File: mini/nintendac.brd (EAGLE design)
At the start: 30 x 45 mm, 30 parts, among them IC1 STM32F10XCXT6, IC2 REG1117, IC3 24C64ST, X1 USB-MICROB

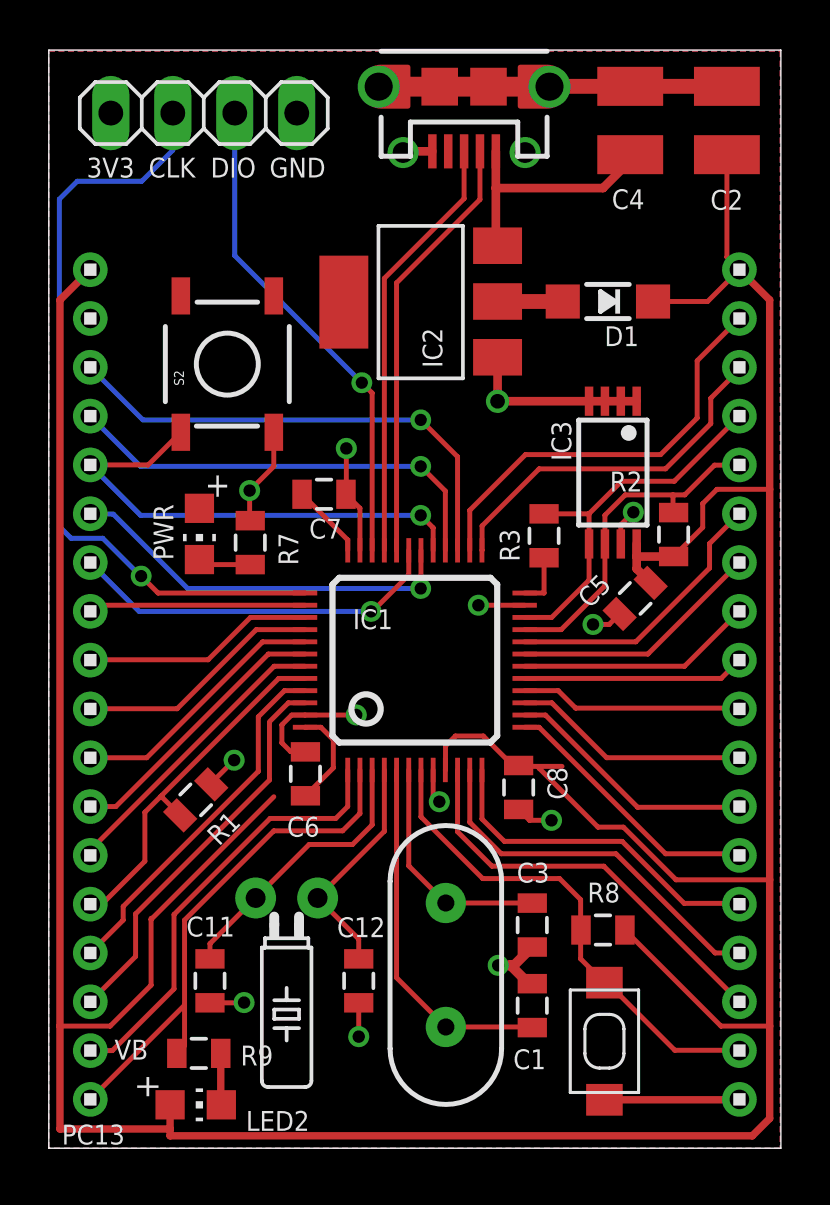
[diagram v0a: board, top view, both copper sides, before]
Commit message: updated mini layout
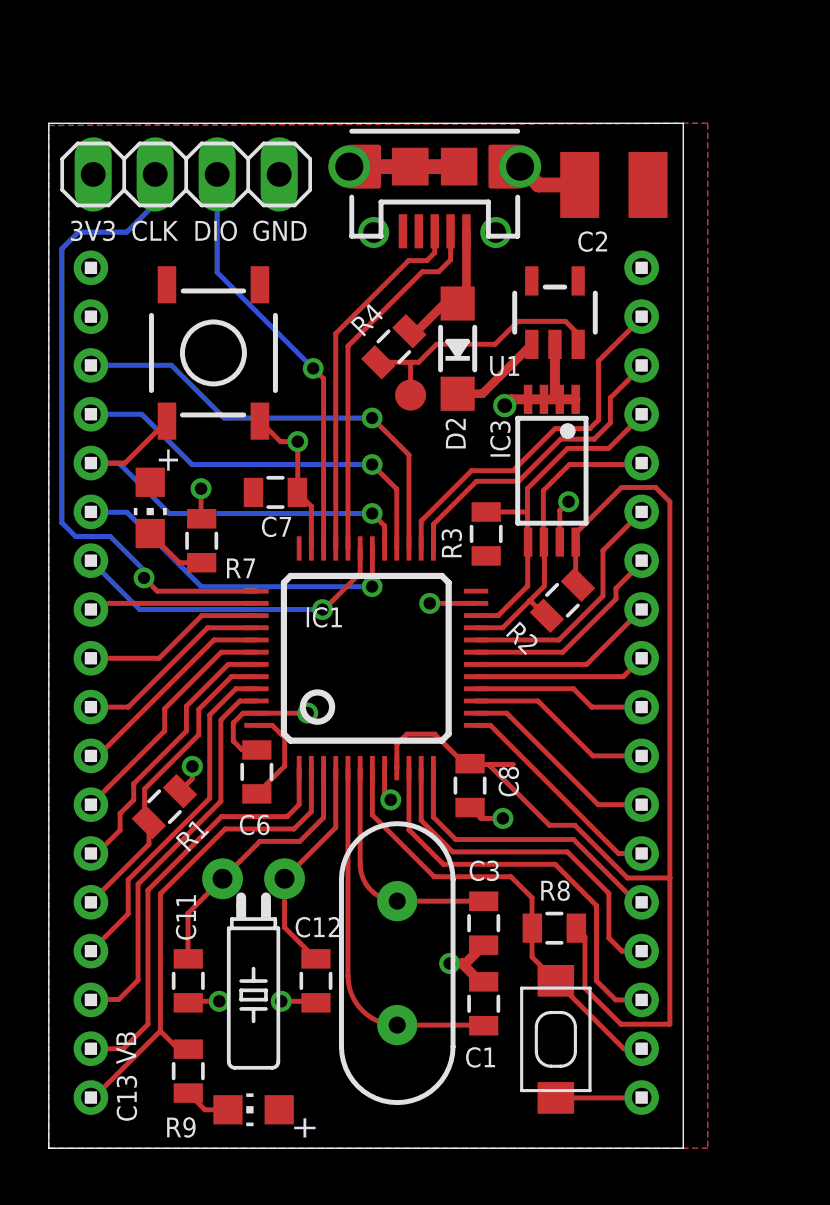
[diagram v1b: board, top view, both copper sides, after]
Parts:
- removed C4: (no value), backplane:C1210
- removed C5: (no value), backplane:0805
- removed D1: MBR120, microbuilder:SOD-123
- removed IC2: REG1117, backplane:SOT223
- added D2: MBR120, microbuilder:SOD-123
- added R4: (no value), SparkFun-Passives:0805
- added TP1: TEST-POINT3X5, SparkFun-Passives:PAD.03X.05
- added U1: (no value), Adafruit Feather M0 Adalogger:SOT23-5
- moved C2 5.33 mm to (23.2, 39.5), turned to 180 degrees
- moved R2 5.29 mm to (21.0, 22.5), turned to 45 degrees
- moved U$2 4.01 mm to (24.3, 27.1)
- moved X1 3.49 mm to (15.8, 40.2)
- moved JP1 2.62 mm to (5.63, 39.9)
- moved IC3 2.50 mm to (20.6, 27.8)
- moved LED2 2.38 mm to (8.39, 1.57), turned to 90 degrees
- moved R3 2.37 mm to (17.9, 25.2)
- moved PWR 2.28 mm to (4.16, 26.2)
- moved C1 1.99 mm to (17.8, 5.92)
- moved C3 1.99 mm to (17.8, 9.22)
- moved C8 1.99 mm to (17.3, 14.9)
- moved IC1 1.99 mm to (13.0, 20.1)
- moved R7 1.99 mm to (6.26, 24.9)
- moved R8 1.99 mm to (20.7, 9.02)
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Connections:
- new net N$31: D2.C, U1.1
- net +3V3: now also U1.5; no longer C5.1, D1.C
- net GND: now also U1.2; no longer C4.2, C5.2, IC2.1
- net N$2: now also D2.A, R4.2; no longer C4.1, IC2.3
- net N$36: now also R4.1, TP1.P$1, U1.3; no longer D1.A, IC2.2
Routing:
- net +3V3: track 168.8 -> 55.2 mm
- net GND: track 56.8 -> 42.5 mm, vias 13 -> 12
- net N$36: track 2.67 -> 11.0 mm
- net N$9: track 31.6 -> 26.3 mm
- net N$2: track 10.1 -> 5.56 mm
- net N$31: track 0.00 -> 3.88 mm
- net N$8: track 20.3 -> 17.1 mm
- net N$7: track 17.8 -> 15.1 mm
- net N$4: track 17.7 -> 15.1 mm
- net N$43: track 20.3 -> 17.9 mm
- net N$39: track 17.3 -> 15.1 mm
- net N$3: track 14.9 -> 12.8 mm
- net N$38: track 14.9 -> 12.9 mm
- net N$14: track 10.4 -> 8.34 mm
- net N$1: track 20.4 -> 18.4 mm
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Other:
- board size 30 x 45 mm -> 26 x 42 mm
- board text added: "C13"
- board text removed: "PC13"
